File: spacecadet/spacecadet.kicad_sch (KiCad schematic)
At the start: 41 parts, among them J1 Conn_01x05_Male, SW1 SW_PUSH, T2 USBD-, T3 USBD+, U1 MIC5504-3.3YM5-TR, U2 GD32F303CGT6, U4 SRV05-4HTG

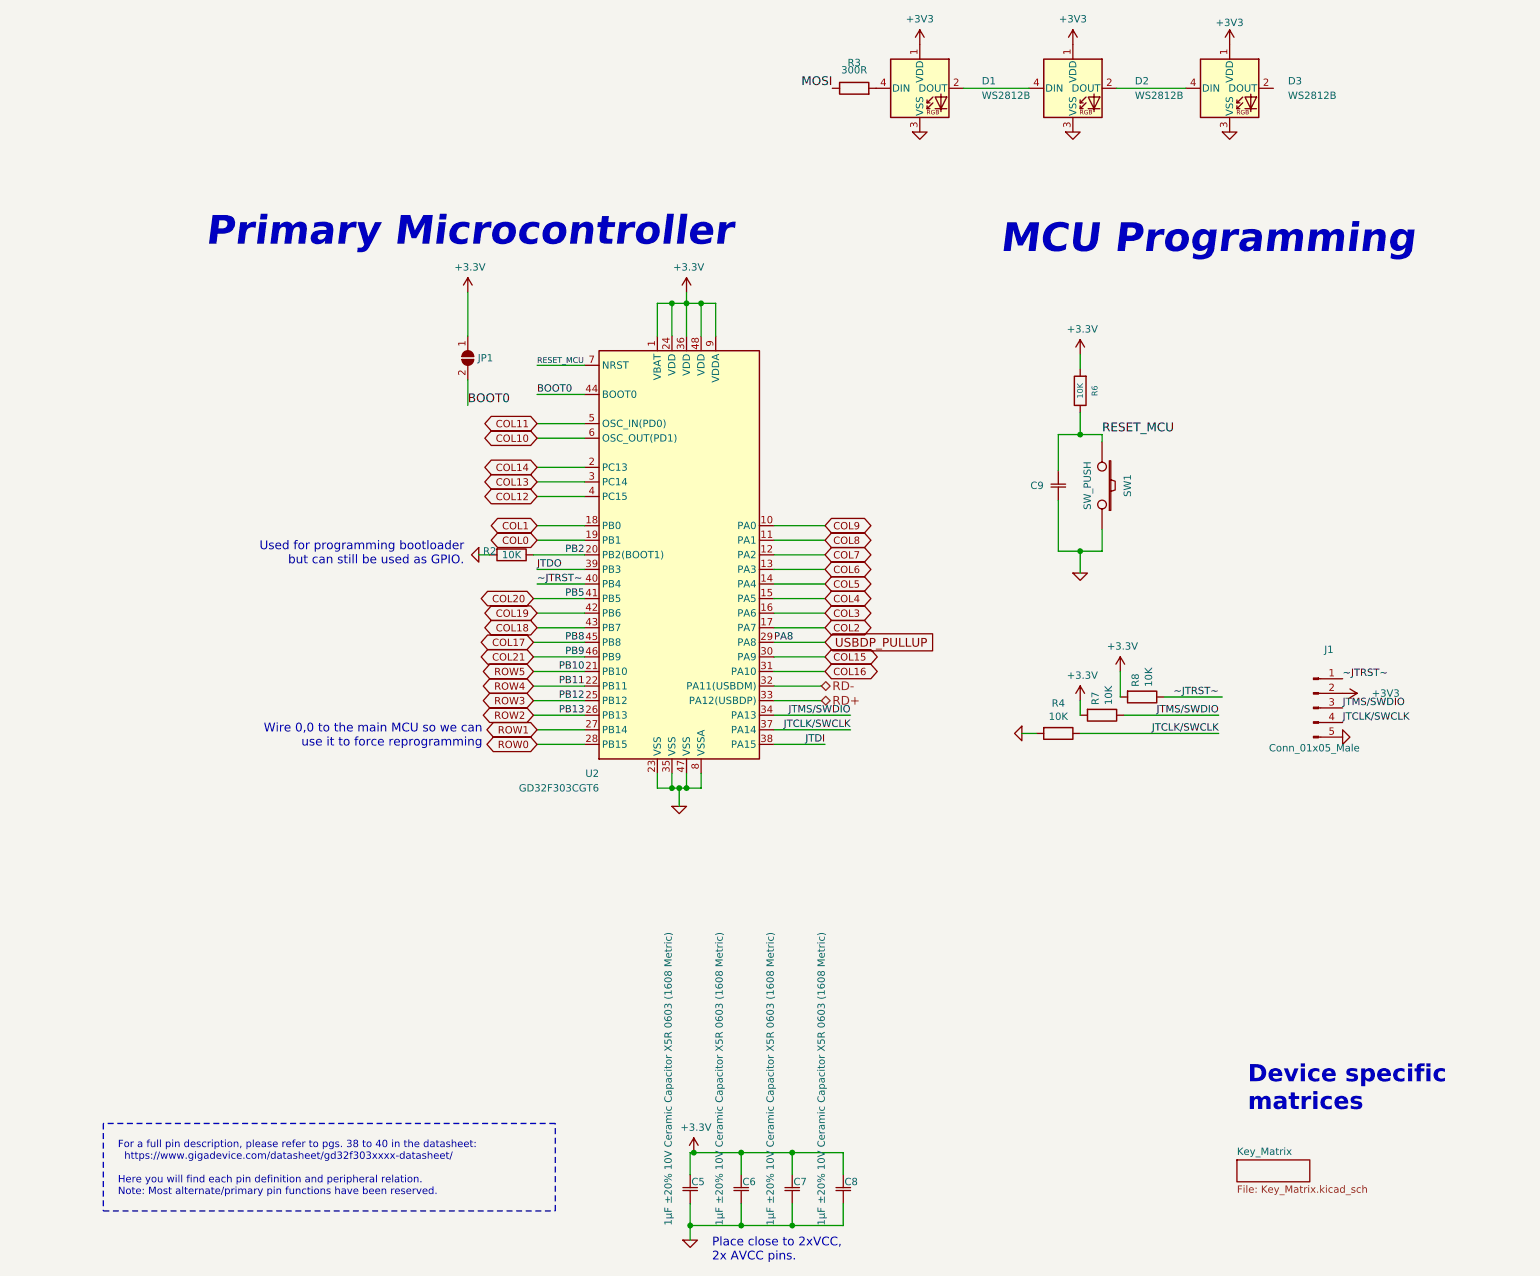
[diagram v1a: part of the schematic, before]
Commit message: Fix boot0 jumper design
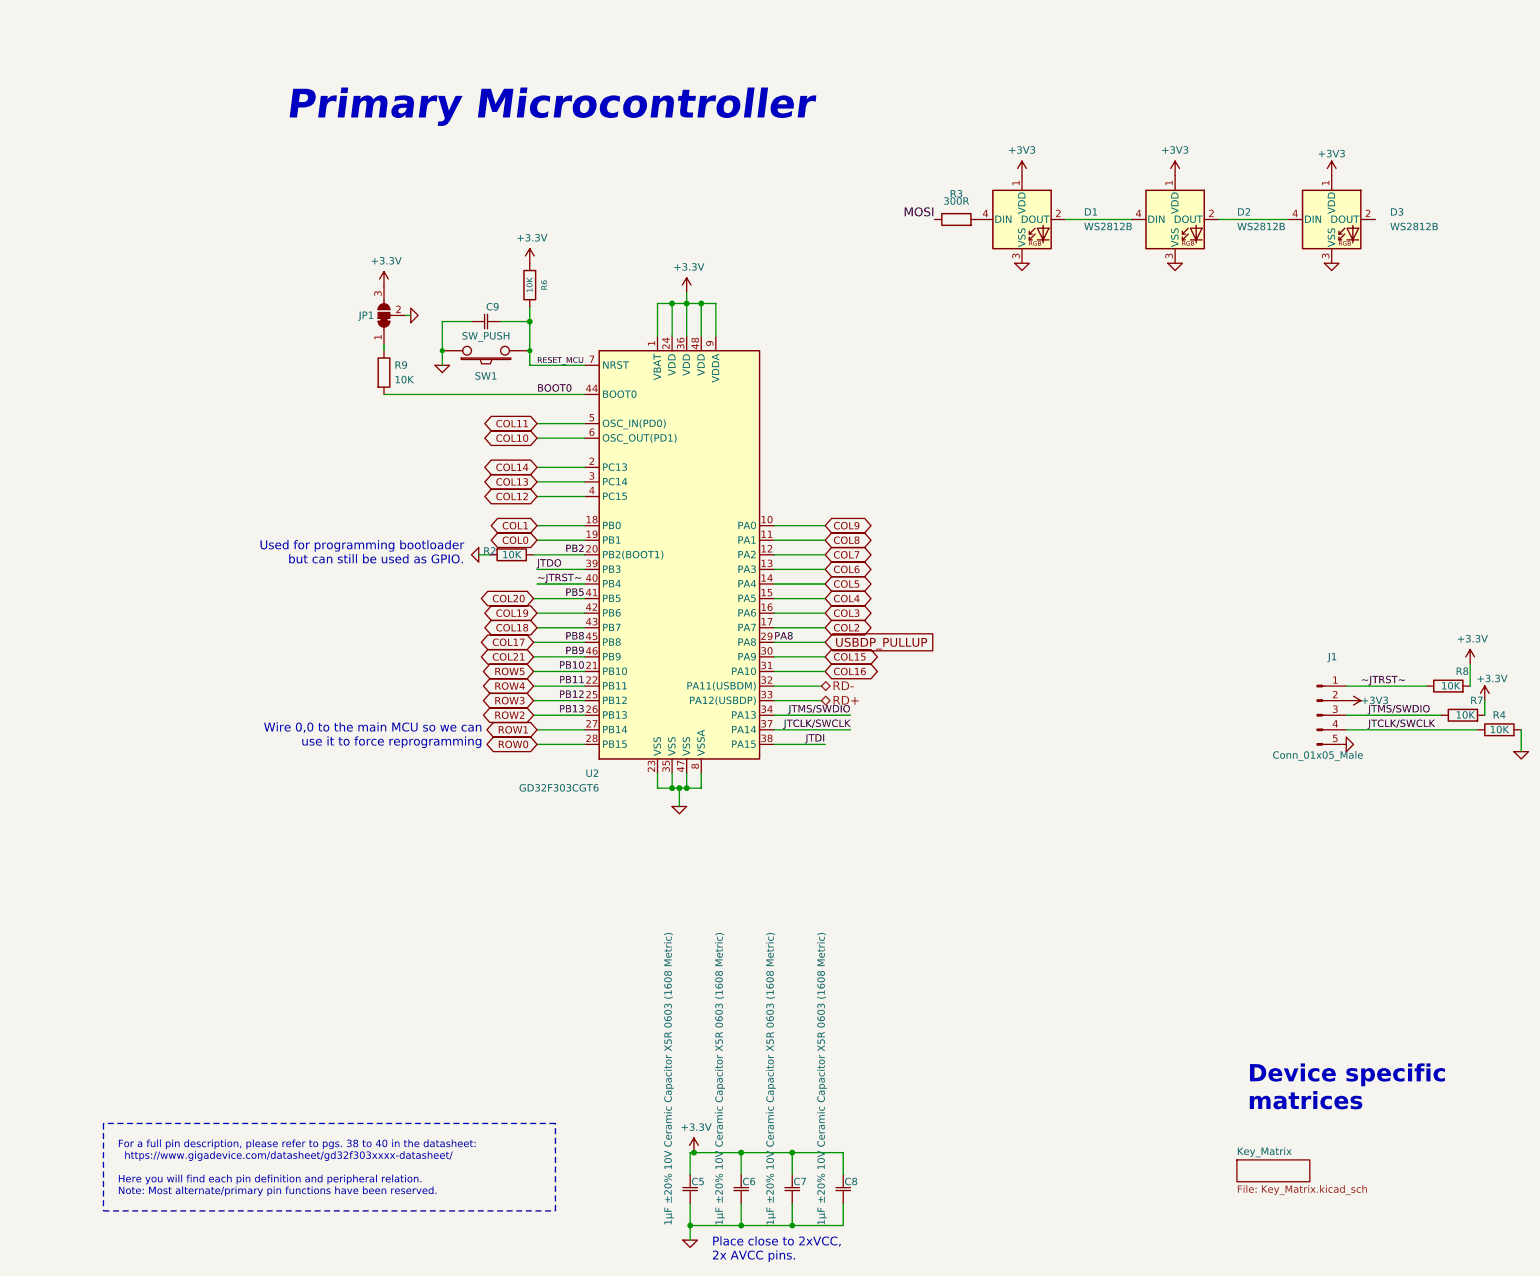
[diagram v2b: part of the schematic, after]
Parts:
- added R9: 10K, Resistor_SMD:R_0603_1608Metric, symbol Device:R
- JP1: footprint Jumper:SolderJumper-2_P1.3mm_Bridged_RoundedPad1.0x1.5mm -> Jumper:SolderJumper-3_P1.3mm_Bridged12_Pad1.0x1.5mm; symbol Jumper:SolderJumper_2_Open -> Jumper:SolderJumper_3_Bridged12; now in the parts list
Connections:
- net +3V3: now also JP1.3 (B); no longer JP1.1 (A)
- net BOOT0: now also R9.2; no longer JP1.2 (B)
- net GND: now also JP1.2 (C)
- new net: JP1.1 (A), R9.1
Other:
- note removed: "MCU Programming"
- moved on the sheet: C9, D1, D2, D3, J1, R3, R4, R6, R7, R8, SW1
